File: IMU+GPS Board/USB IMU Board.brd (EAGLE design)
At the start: 75 x 72 mm, 36 parts, among them IC1 MCP1703CB, J1 CON_HEADER_PRG_AVR_ICSP-SMD, Y1 16 MHz

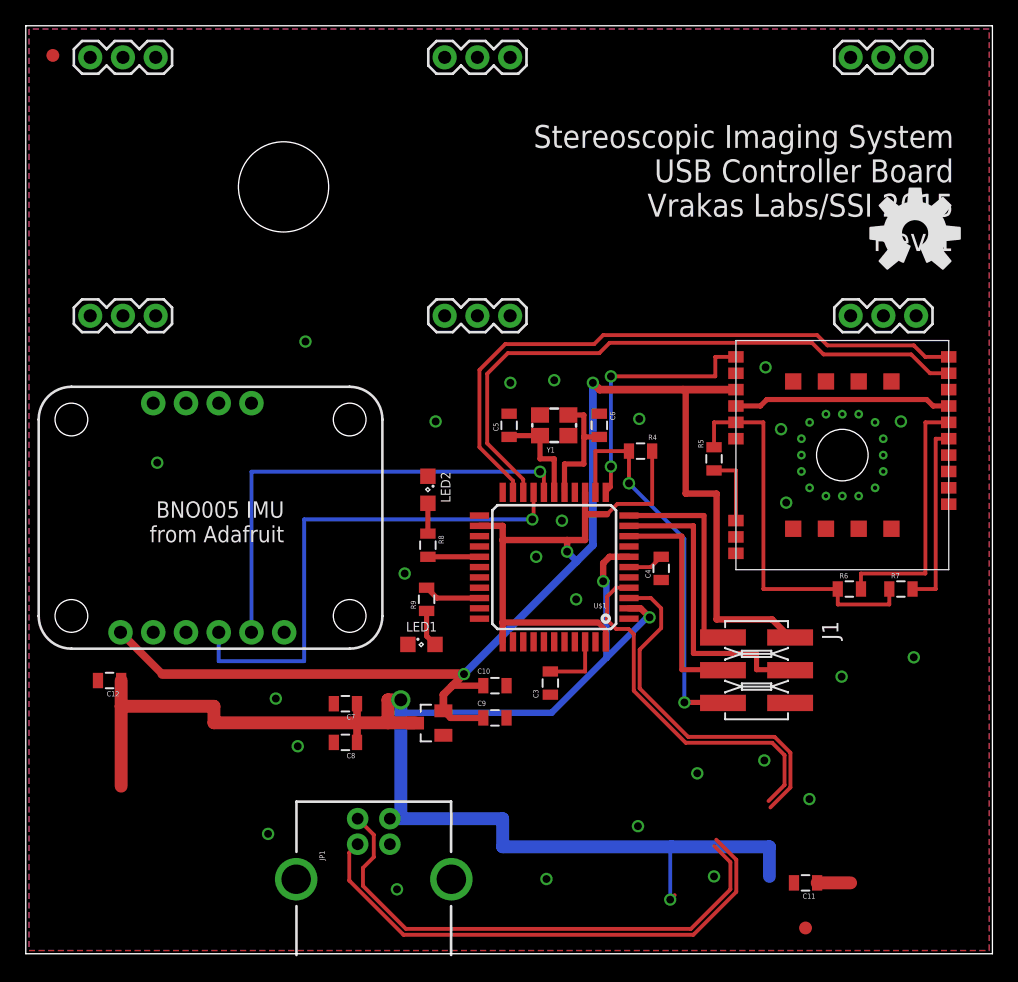
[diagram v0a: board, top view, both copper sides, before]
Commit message: First Round of new board
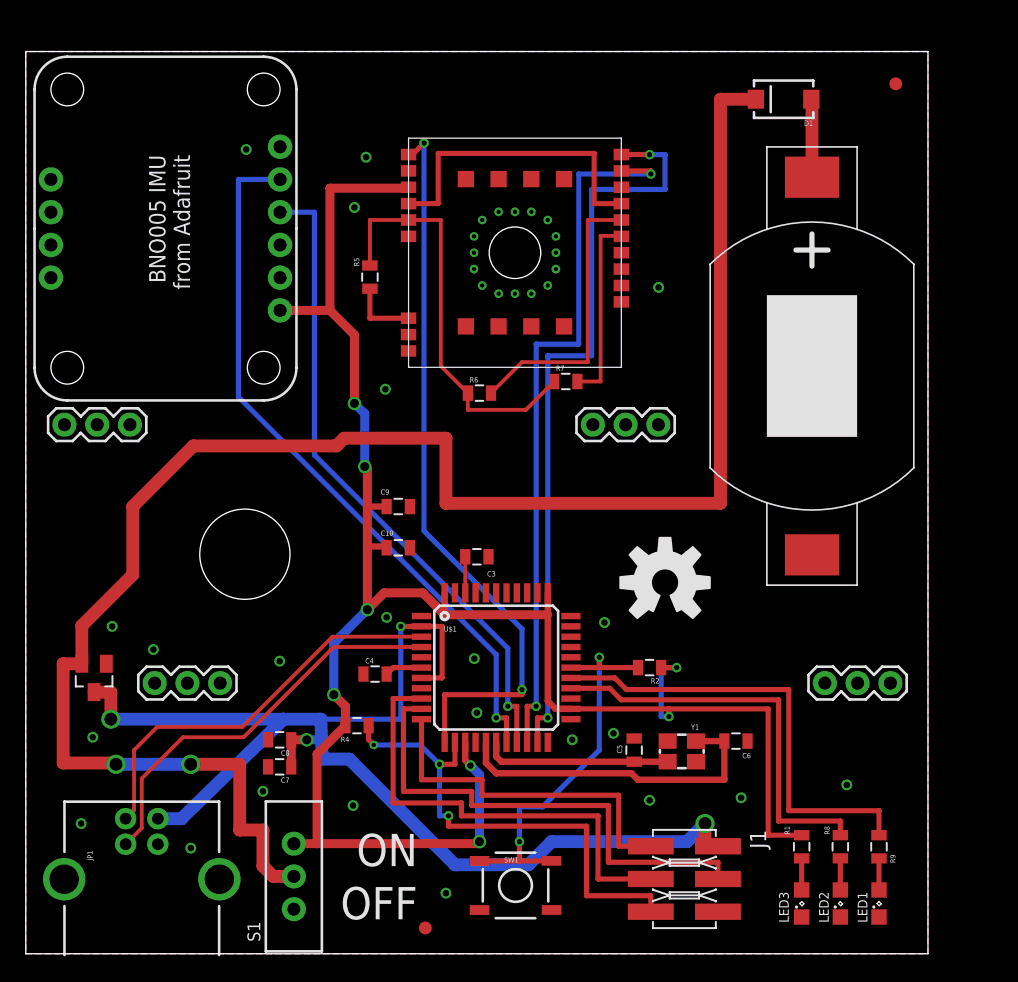
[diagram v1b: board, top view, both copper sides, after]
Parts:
- removed C11, C12: (no value), SparkFun-Capacitors:0805
- removed JP2, JP6: (no value), SparkFun-Connectors:1X03
- added D1: (no value), SparkFun-DiscreteSemi:SMA-DIODE
- added LED3: BLUE, led:SML0805
- added R1: 220, SparkFun-Resistors:0805
- added R2: 10K, SparkFun-Resistors:0805
- added S1: (no value), SparkFun-Electromechanical:SWITCH-SPDT
- added SW1: (no value), SparkFun-Electromechanical:TACTILE-SWITCH-SMD
- added U$3: 3V, NASA Parts Lib:BU2032SM-G
- Y1: value 16 MHz -> 16Mhz
- moved U$7 65.4 mm to (67.5, 67.5)
- moved FRAME1 63.5 mm to (61.1, 17.2)
- moved U$4 46.4 mm to (21.0, 69.6), turned to 180 degrees
- moved LED2 45.3 mm to (63.2, 3.90), turned to 90 degrees
- moved JP7 41.0 mm to (62.0, 21.0)
- moved LED1 40.8 mm to (66.2, 3.90), turned to 90 degrees
- moved R9 40.0 mm to (66.2, 8.30)
- moved R8 39.6 mm to (63.2, 8.30), turned to 90 degrees
- moved JP4 34.8 mm to (44.0, 41.0)
- moved U$9 33.3 mm to (49.6, 28.8)
- moved R6 32.5 mm to (35.2, 43.5)
- moved R4 30.6 mm to (25.7, 17.7), turned to 0 degrees
- moved R7 30.6 mm to (41.9, 44.4)
- moved R5 30.2 mm to (26.7, 52.5)
- moved U$2 29.9 mm to (29.7, 45.5)
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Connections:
- removed net N$14: R9.2, U$1.31
- removed net N$15: R8.2, U$1.27
- removed net USB2_N: U$1.3
- removed net USB2_P: U$1.4
- new net 3V3IN: D1.C, IC1.2, S1.2
- new net LED1: R9.2, U$1.27
- new net LED2: R8.2, U$1.26
- new net N$4: LED3.A, R1.2
- new net N$5: D1.A, U$3.PVCC
- new net PWRBTN: R2.2, SW1.1, SW1.2, U$1.28
- net DIN_N: now also U$1.3
- net DIN_P: now also U$1.4
- net GND: now also LED3.C, SW1.3, SW1.4, U$3.PGND; no longer C11.2, C12.2
- net VCC: now also R1.1, R2.1, S1.3; no longer IC1.2, J1.2
- net VUSB: now also J1.2; no longer C11.1, C12.1
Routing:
- net 3V3IN: track 0.00 -> 136.2 mm, vias 0 -> 2
- net GPS_RST: track 20.4 -> 57.2 mm
- net LED1: track 0.00 -> 35.6 mm
- net LED2: track 0.00 -> 31.8 mm
- net PWRBTN: track 0.00 -> 31.0 mm, vias 0 -> 2
- net USB2_P: track 28.6 -> 0.00 mm
- net USB2_N: track 28.4 -> 0.00 mm
- net VUSB: track 122.6 -> 99.5 mm
- net SCL: track 36.8 -> 56.0 mm
- net SCK: track 17.7 -> 36.2 mm
- net N$2: track 9.90 -> 25.8 mm
- net MOSI: track 23.7 -> 39.0 mm
- net VCC: track 143.6 -> 155.7 mm, vias 3 -> 8
- net SDA: track 39.7 -> 50.7 mm
- net MISO: track 16.8 -> 27.7 mm
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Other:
- board size 75 x 72 mm -> 70 x 70 mm
- board text added: "ON OFF"
- board text added: "Stereoscopic Imaging System USB Sensor Board Vrakas Labs/SSI 2016 Rev.2"
- board text removed: "Stereoscopic Imaging System USB Controller Board Vrakas Labs/SSI 2015 Rev.1"
